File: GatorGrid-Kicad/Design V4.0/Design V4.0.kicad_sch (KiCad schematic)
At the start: 30 parts, among them J1 Battery-Connector, J2 Conn_01x20_Pin, J3 Conn_01x20_Pin, J4 Conn_01x20_Pin, J5 Conn_01x20_Pin, J7 Conn_01x03, Q3 2N3904, Q4 2N3904, SW1 SW_SPST, U1 TP4056

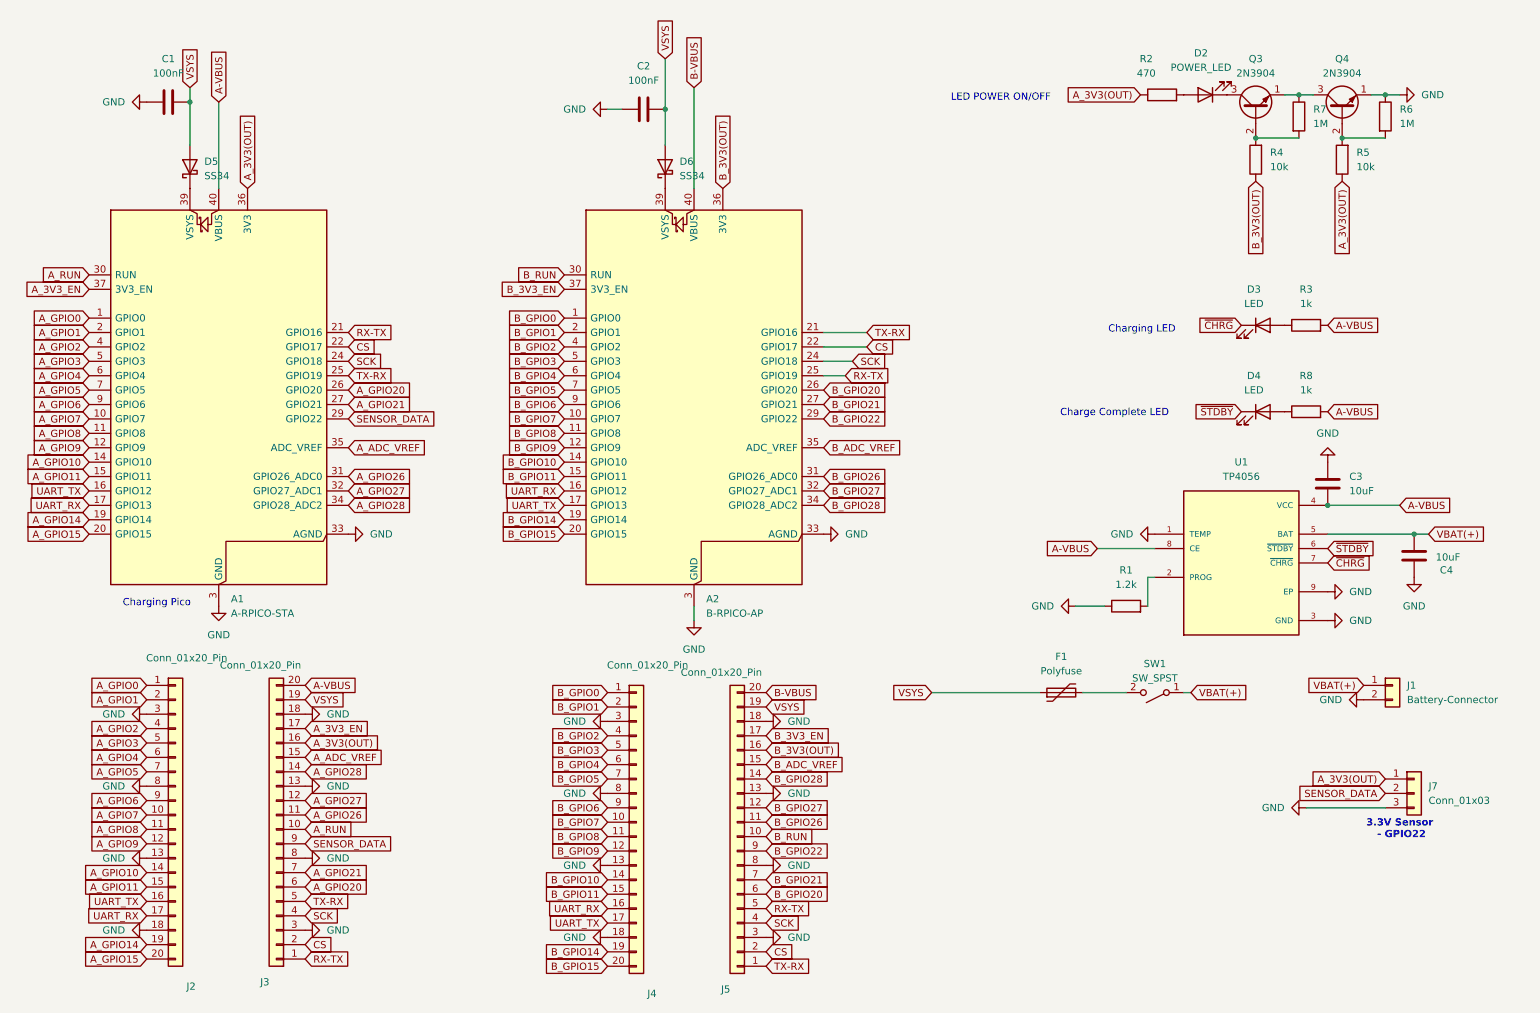
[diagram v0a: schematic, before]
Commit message: Finished PCB design for V4.0
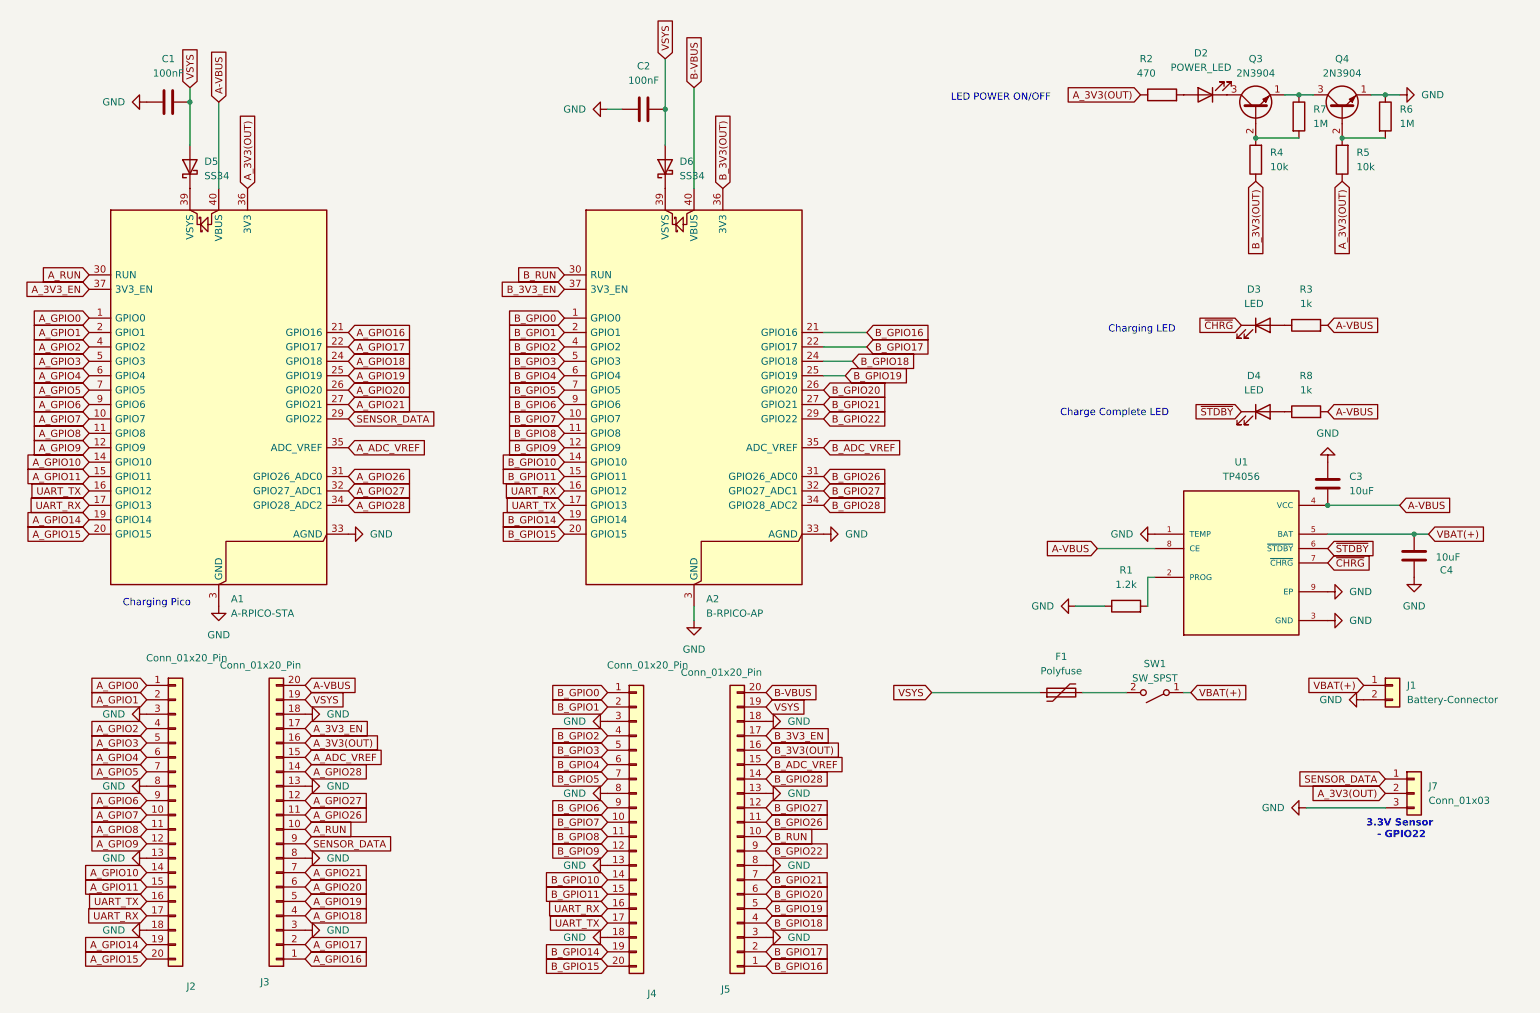
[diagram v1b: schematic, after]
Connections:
- net A_3V3(OUT): now also J7.2 (Pin_2); no longer J7.1 (Pin_1)
- net SENSOR_DATA: now also J7.1 (Pin_1); no longer J7.2 (Pin_2)
- net CS renamed A_GPIO17
- net A_GPIO17: no longer A2.22 (GPIO17), J5.2 (Pin_2)
- net RX-TX renamed A_GPIO16
- net A_GPIO16: no longer A2.25 (GPIO19), J5.5 (Pin_5)
- net SCK renamed A_GPIO18
- net A_GPIO18: no longer A2.24 (GPIO18), J5.4 (Pin_4)
- net TX-RX renamed A_GPIO19
- net A_GPIO19: no longer A2.21 (GPIO16), J5.1 (Pin_1)
- new net B_GPIO16: A2.21 (GPIO16), J5.1 (Pin_1)
- new net B_GPIO17: A2.22 (GPIO17), J5.2 (Pin_2)
- new net B_GPIO18: A2.24 (GPIO18), J5.4 (Pin_4)
- new net B_GPIO19: A2.25 (GPIO19), J5.5 (Pin_5)

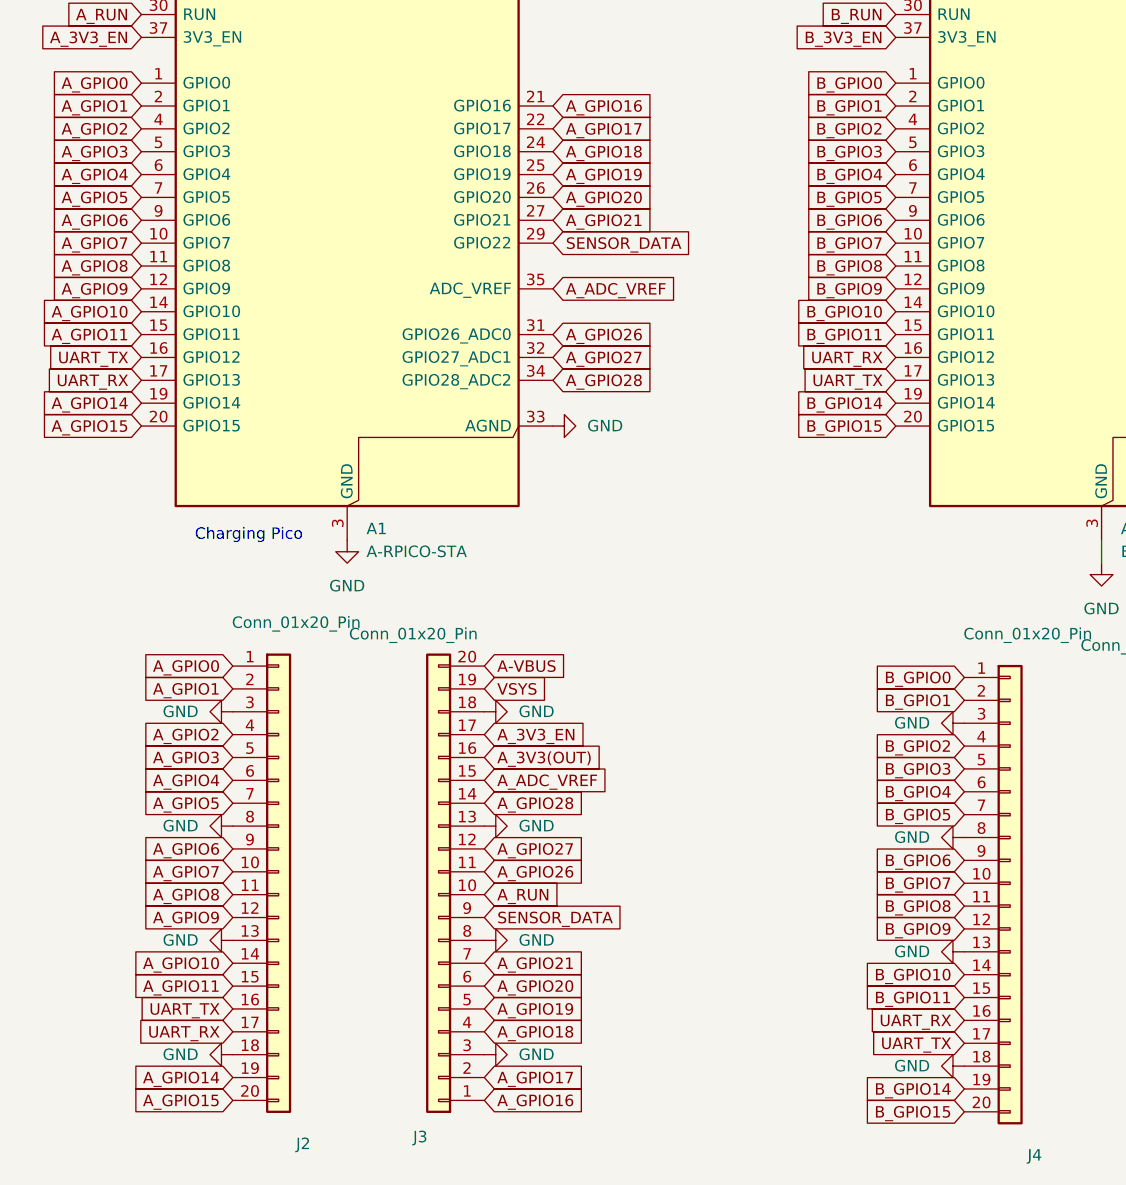
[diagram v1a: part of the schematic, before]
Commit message: Finihsed design
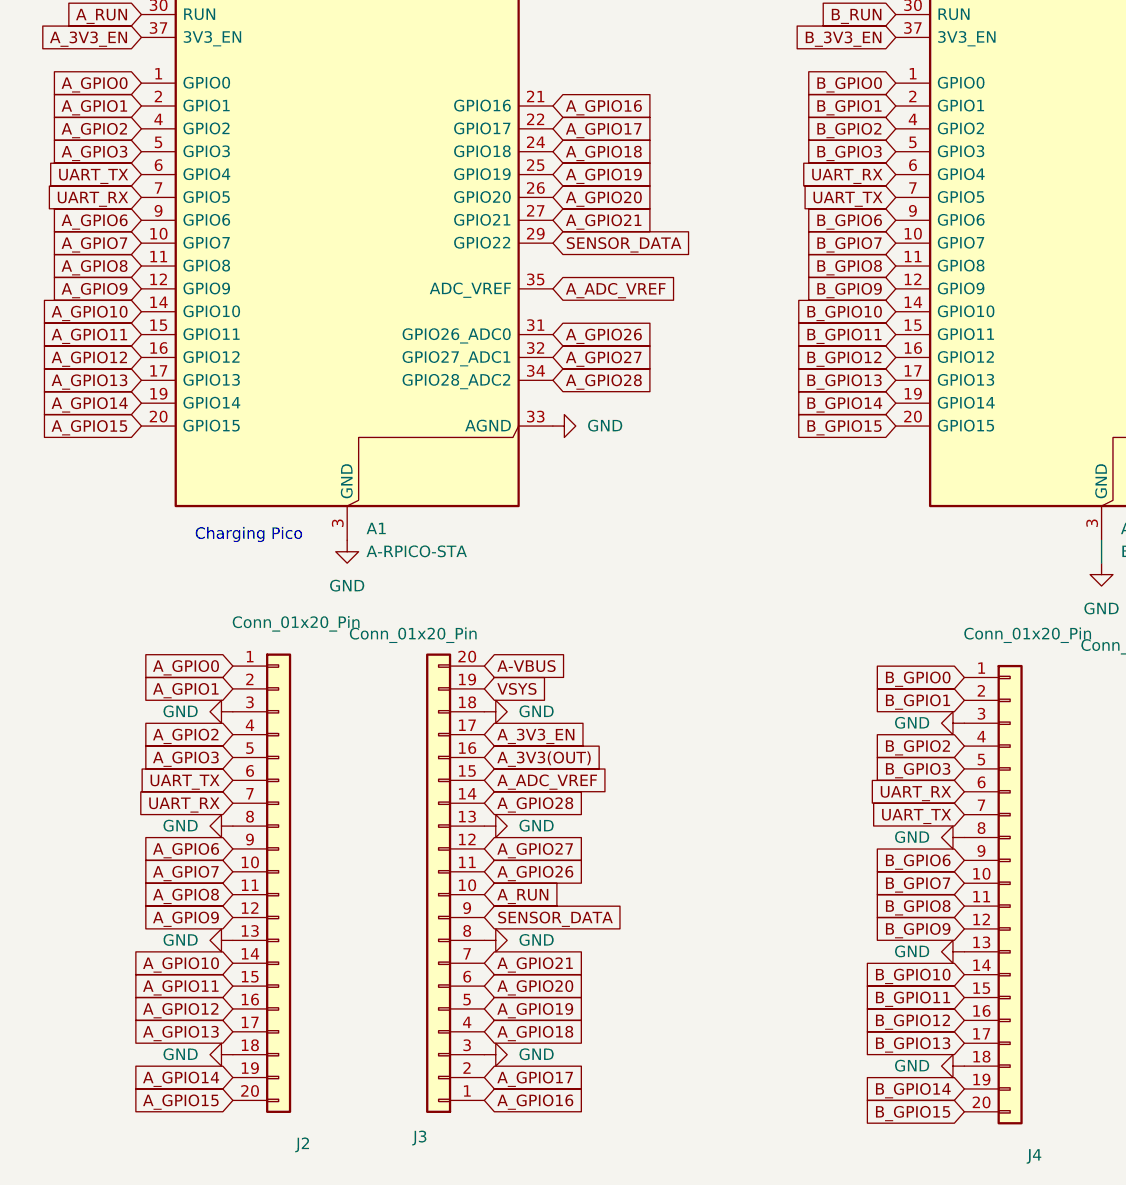
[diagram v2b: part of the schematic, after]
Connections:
- net A_GPIO4 is gone; now on net UART_TX: A1.6 (GPIO4), J2.6 (Pin_6)
- net A_GPIO5 is gone; now on net UART_RX: A1.7 (GPIO5), J2.7 (Pin_7)
- net B_GPIO4 is gone; now on net UART_RX: A2.6 (GPIO4), J4.6 (Pin_6)
- net B_GPIO5 is gone; now on net UART_TX: A2.7 (GPIO5), J4.7 (Pin_7)
- net UART_RX: no longer A1.17 (GPIO13), A2.16 (GPIO12), J2.17 (Pin_17), J4.16 (Pin_16)
- net UART_TX: no longer A1.16 (GPIO12), A2.17 (GPIO13), J2.16 (Pin_16), J4.17 (Pin_17)
- new net A_GPIO12: A1.16 (GPIO12), J2.16 (Pin_16)
- new net A_GPIO13: A1.17 (GPIO13), J2.17 (Pin_17)
- new net B_GPIO12: A2.16 (GPIO12), J4.16 (Pin_16)
- new net B_GPIO13: A2.17 (GPIO13), J4.17 (Pin_17)
